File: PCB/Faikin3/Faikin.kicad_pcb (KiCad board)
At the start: 2 copper layers, 70 x 70 mm, 28 parts, among them J1 1x5, J2 Prog, Q3 PMF250XNEX, U1 ESP32-PICO-MINI-02, U3 MD8942, U4 Barcode

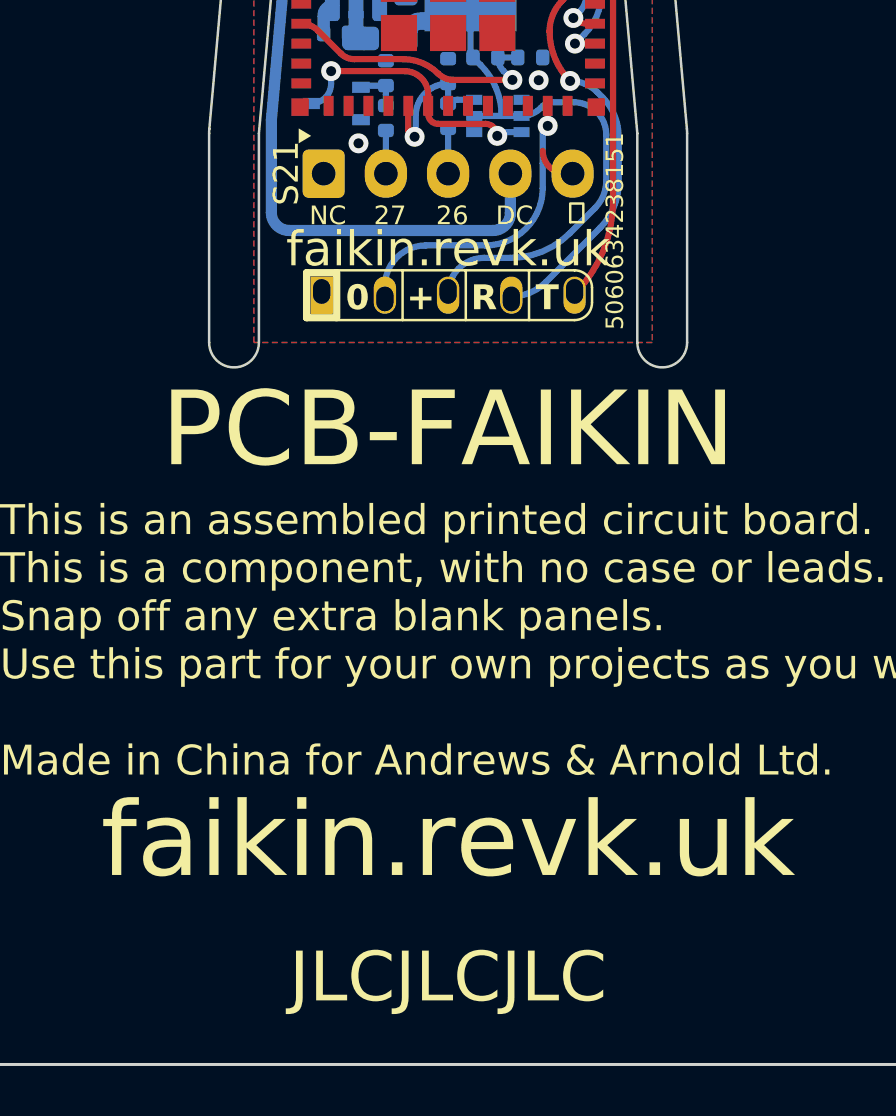
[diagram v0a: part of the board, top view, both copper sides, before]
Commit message: Order
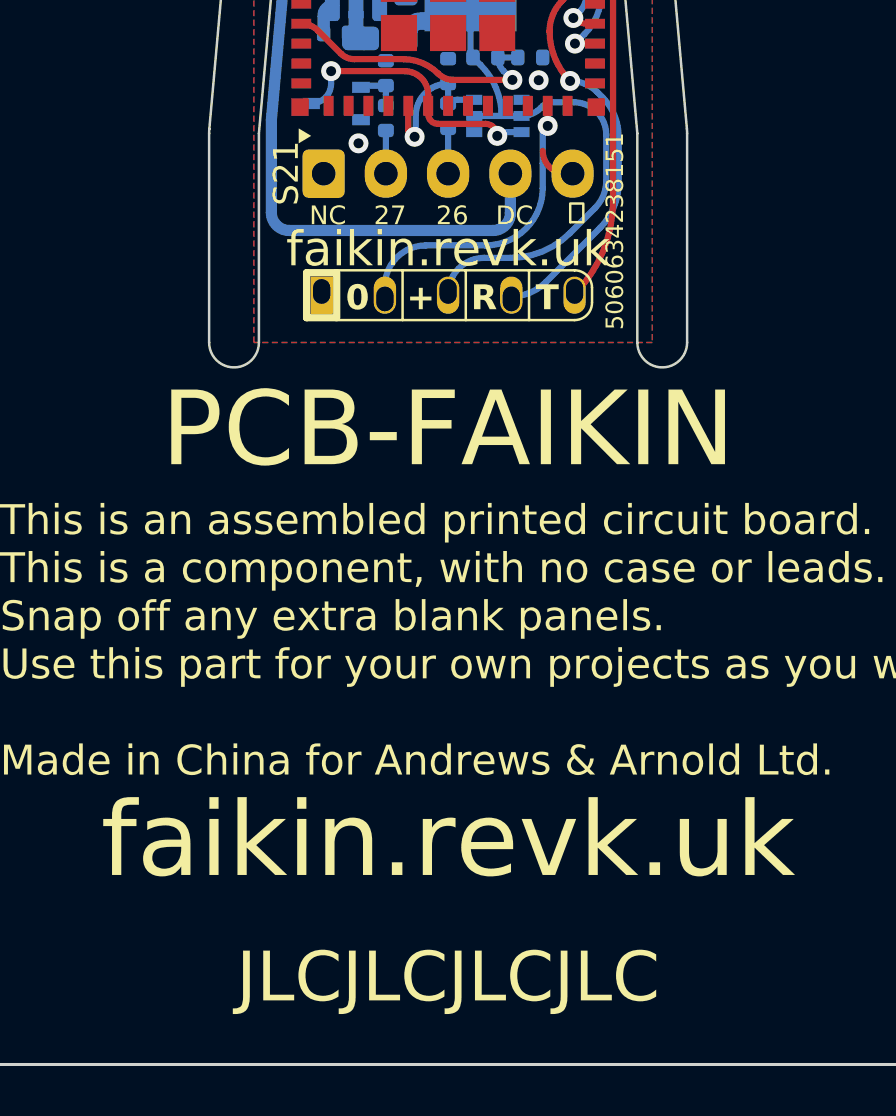
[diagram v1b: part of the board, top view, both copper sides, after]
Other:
- board text removed: "JLCJLCJLC"
